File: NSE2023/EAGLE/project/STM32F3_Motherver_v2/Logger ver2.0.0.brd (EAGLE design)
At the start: 35 x 45 mm, 24 parts

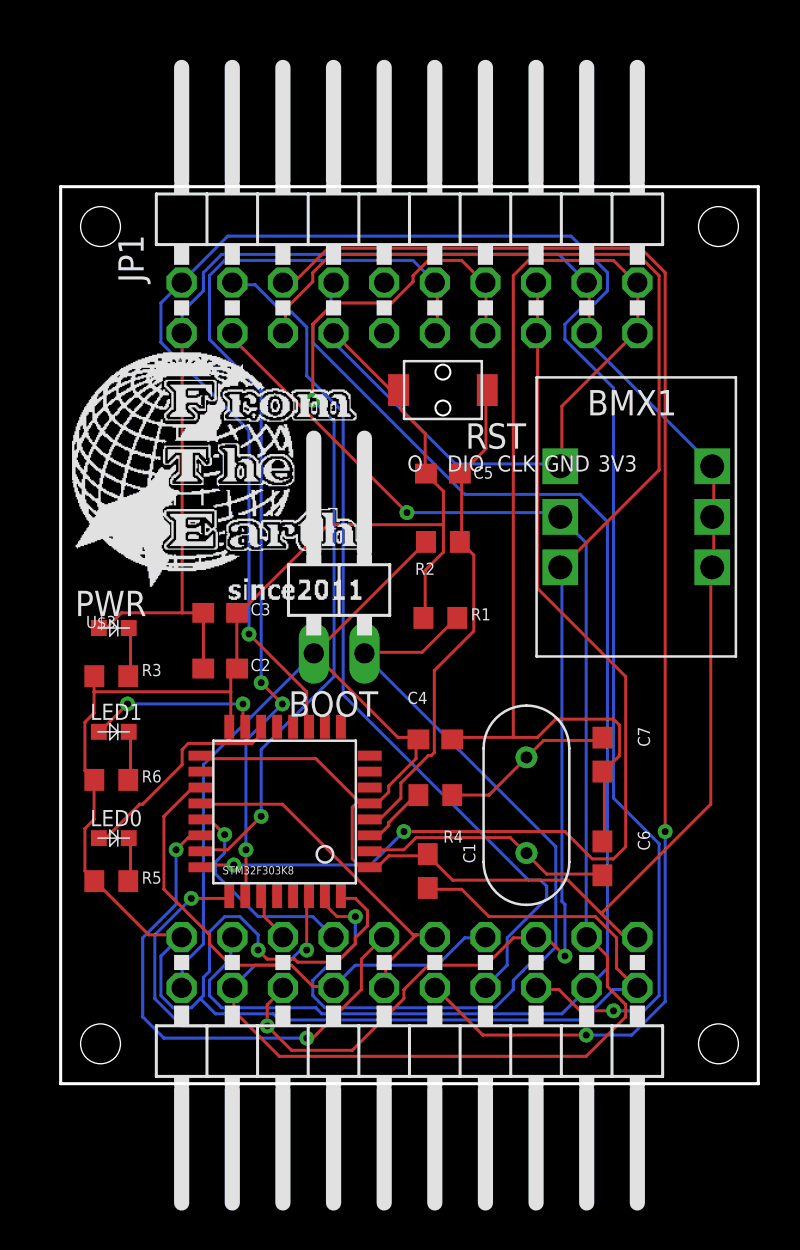
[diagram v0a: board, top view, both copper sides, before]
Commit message: create final board NSE2023
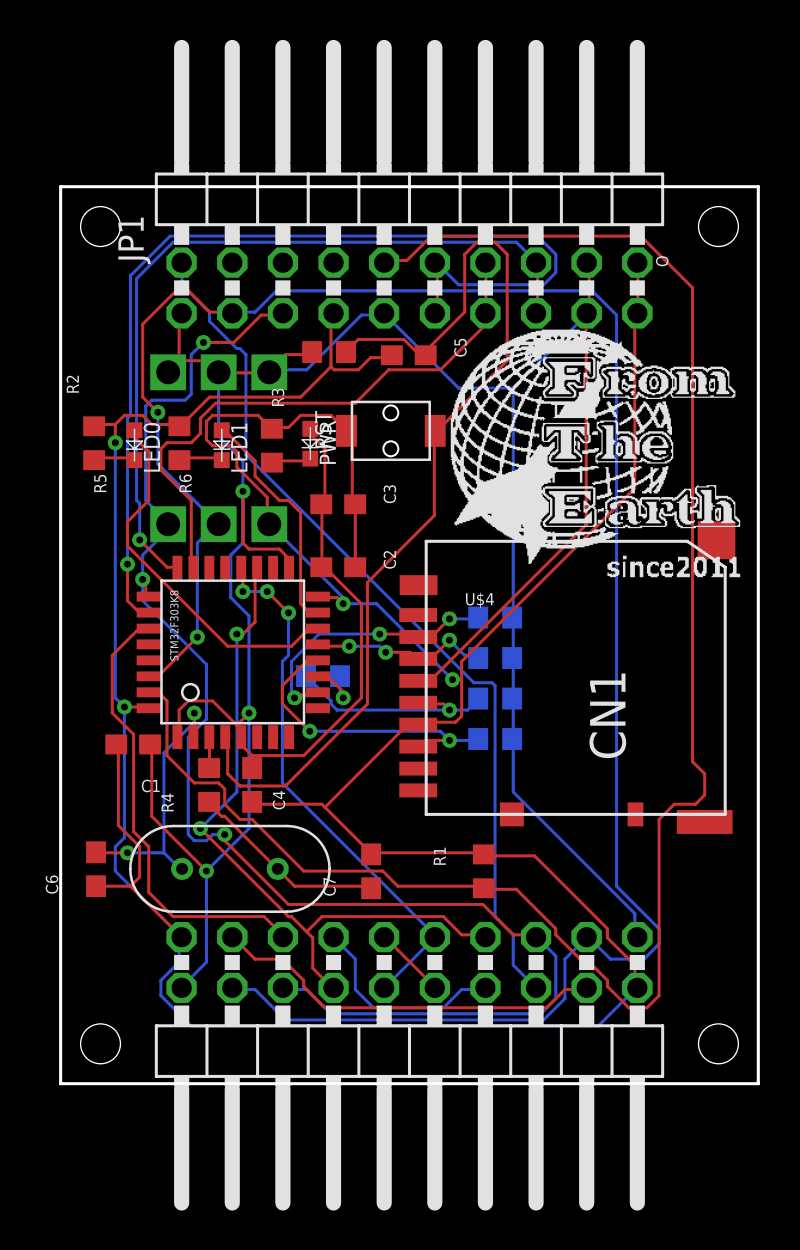
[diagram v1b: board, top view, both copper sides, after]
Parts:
- removed BOOT: (no value), pinhead:1X02/90
- removed U$3: F.T.E.LOGO, logo:LOGO
- added CN1: DM3AT, microSD:DM3AT
- added R10, R7, R8, R9: 10k, rcl:R0603
- added R11: 100, rcl:R0603
- added U$4: F.T.E.LOGO, logo:LOGO
- moved C6 25.4 mm to (1.77, 10.8), turned to 270 degrees
- moved R5 22.0 mm to (1.68, 32.1), turned to 270 degrees
- moved LED0 19.7 mm to (3.70, 32.0), turned to 270 degrees
- moved R6 17.2 mm to (5.96, 32.1), turned to 270 degrees
- moved C1 16.1 mm to (3.64, 17.0), turned to 180 degrees
- moved LED1 15.4 mm to (8.08, 32.0), turned to 270 degrees
- moved CRY1 15.2 mm to (8.49, 10.8), turned to 180 degrees
- moved R3 14.1 mm to (10.6, 32.0), turned to 270 degrees
- moved PWR 13.5 mm to (12.5, 32.1), turned to 270 degrees
- moved C7 13.0 mm to (15.6, 10.7), turned to 90 degrees
- moved R1 12.9 mm to (21.2, 10.7), turned to 90 degrees
- moved BMX1 12.4 mm to (14.9, 26.9), flipped to the bottom, turned to 90 degrees
- moved R4 11.4 mm to (7.45, 15.0), turned to 90 degrees
- moved R2 11.1 mm to (13.5, 36.7)
- moved C4 9.47 mm to (9.61, 15.0), turned to 270 degrees
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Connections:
- new net MISO: CN1.DAT0, R10.1, U$1.PA6/SPI1_MISO
- new net MOSI: CN1.CMD, R8.1, U$1.PA7/SPI1_MOSI
- new net N$11: JP3.17, JP3.4
- new net N$7: CN1.CLK, R11.2, R9.1
- new net NSS: CN1.CD/DAT3, R7.1, U$1.PA4/SPI1_NSS
- new net SCK: R11.1, U$1.PA5/SPI1_SCK
- net +3V3: now also CN1.VDD, JP1.9, R10.2, R7.2, R8.2, R9.2; no longer BOOT.1
- net +5V: no longer JP3.17, JP3.4
- net BIT1: now also JP3.10; no longer U$1.PA12/CAN_TX
- net BIT2: now also JP3.8; no longer U$1.PA11/CAN_RX
- net BOOT0: now also JP1.10; no longer BOOT.2
- net FPRAW: no longer JP3.10
- net GND: now also CN1.VSS
- net PWM: no longer U$1.PA5/SPI1_SCK
- net SW: no longer JP3.8
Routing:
- net FPRAW: track 70.2 -> 0.00 mm, vias 2 -> 0
- net +5V: track 69.1 -> 0.00 mm
- net PWM: track 95.3 -> 44.4 mm, vias 2 -> 0
- net SW: track 44.4 -> 0.00 mm
- net BOOT0: track 45.3 -> 89.3 mm, vias 1 -> 0
- net SDA: track 76.8 -> 105.2 mm
- net NRST: track 25.1 -> 49.6 mm
- net BIT1: track 26.1 -> 3.60 mm, vias 2 -> 0
- net FP_CHECKER: track 2.52 -> 22.7 mm
- net N$11: track 0.00 -> 19.9 mm
- net SCL: track 92.8 -> 73.3 mm
- net MISO: track 0.00 -> 15.5 mm, vias 0 -> 2
- net SWDIO: track 43.6 -> 29.1 mm, vias 2 -> 0
- net SWCLK: track 53.2 -> 39.5 mm, vias 2 -> 1
- net NSS: track 0.00 -> 13.6 mm, vias 0 -> 3
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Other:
- board text removed: "3V3"
- board text removed: "CLK"
- board text removed: "DIO"
- board text removed: "GND"
